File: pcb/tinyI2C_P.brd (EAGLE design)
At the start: 83.2 x 83.2 mm, 218 parts, among them IC1 IC_TTL_74_125, IC10 IC_TTL_74_125, IC11 TPS73618(0.4A), IC12 IC_TTL_74_125, IC13 TPS73618(0.4A), IC14 IC_TTL_74_125, IC15 TPS73618(0.4A), IC16 IC_TTL_74_125, IC2 TPS73618(0.4A), IC3 TPS73618(0.4A), IC4 IC_TTL_74_125, IC5 TPS73618(0.4A), IC6 IC_TTL_74_125, IC7 TPS73618(0.4A), IC8 IC_TTL_74_125, IC9 TPS73618(0.4A), U1 LPC824M201JHI33, U2 LPC824M201JHI33, U3 LPC824M201JHI33, U4 LPC824M201JHI33, U5 LPC824M201JHI33, U6 LPC824M201JHI33, U7 LPC824M201JHI33, U8 LPC824M201JHI33, X1 TSW-112-02-S-S, X10 TSW-102-02-S-S, X11 TSW-106-02-S-S-RA, X12 TSW-112-02-S-S, X13 TSW-112-02-S-S, X14 TSW-102-02-S-S, X15 TSW-102-02-S-S, X16 TSW-106-02-S-S-RA, X17 TSW-112-02-S-S, X18 TSW-112-02-S-S, X19 TSW-102-02-S-S, X2 TSW-106-02-S-S-RA, X20 TSW-102-02-S-S, X21 TSW-106-02-S-S-RA, X22 TSW-112-02-S-S, X23 TSW-112-02-S-S, X24 TSW-102-02-S-S, X25 TSW-102-02-S-S, X26 TSW-106-02-S-S-RA, X27 TSW-112-02-S-S, X28 TSW-112-02-S-S, X29 TSW-102-02-S-S, X3 TSW-112-02-S-S, X30 TSW-102-02-S-S, X31 TSW-106-02-S-S-RA, X32 TSW-112-02-S-S, X33 TSW-112-02-S-S, X34 TSW-102-02-S-S, X35 TSW-102-02-S-S, X36 TSW-106-02-S-S-RA, X37 TSW-112-02-S-S, X38 TSW-112-02-S-S, X39 TSW-102-02-S-S, X4 TSW-102-02-S-S, X40 TSW-102-02-S-S, X5 TSW-102-02-S-S, X6 TSW-106-02-S-S-RA, X7 TSW-112-02-S-S, X8 TSW-112-02-S-S, X9 TSW-102-02-S-S

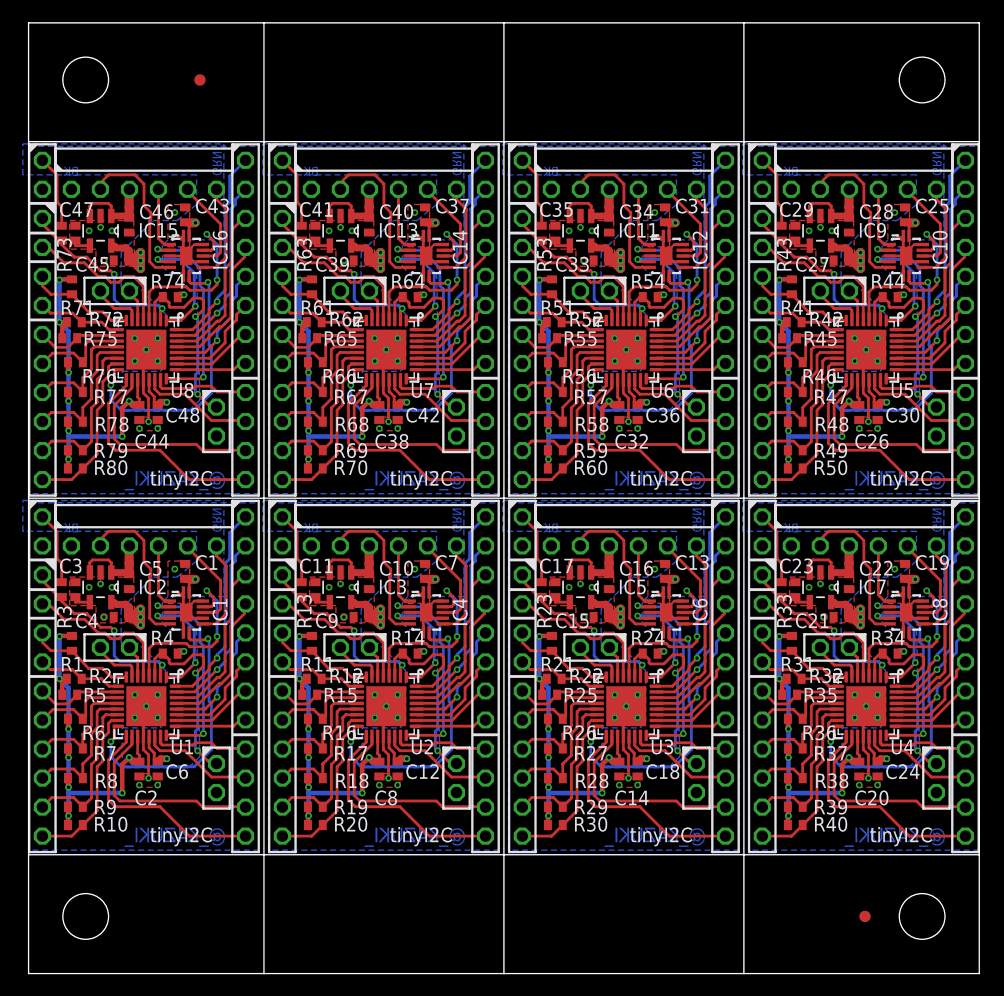
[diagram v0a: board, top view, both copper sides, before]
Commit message: [ PCB ] trace change and panelize
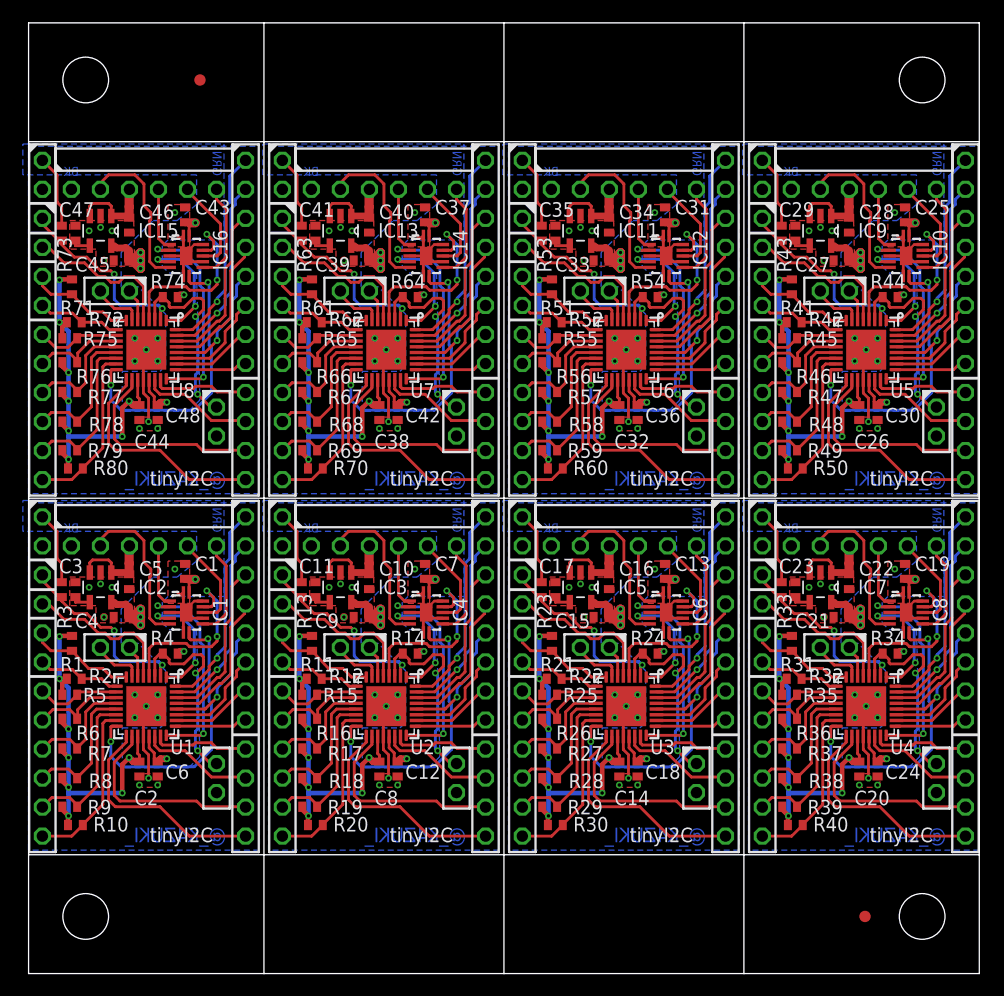
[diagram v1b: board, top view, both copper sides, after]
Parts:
- moved R16 0.50 mm to (24.6, 22.3)
- moved R17 0.50 mm to (24.6, 19.7)
- moved R18 0.50 mm to (24.6, 17.1)
- moved R19 0.50 mm to (24.6, 14.6)
- moved R26 0.50 mm to (45.6, 22.3)
- moved R27 0.50 mm to (45.6, 19.7)
- moved R28 0.50 mm to (45.6, 17.1)
- moved R29 0.50 mm to (45.6, 14.6)
- moved R36 0.50 mm to (66.6, 22.3)
- moved R37 0.50 mm to (66.6, 19.7)
- moved R38 0.50 mm to (66.6, 17.1)
- moved R39 0.50 mm to (66.6, 14.6)
- moved R46 0.50 mm to (66.6, 53.5)
- moved R47 0.50 mm to (66.6, 50.9)
- moved R48 0.50 mm to (66.6, 48.3)
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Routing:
- net 1.8V7: track 53.9 -> 54.7 mm
- net 1.8V6: track 53.9 -> 54.7 mm
- net 1.8V4: track 53.9 -> 54.7 mm
- net 1.8V5: track 53.9 -> 54.7 mm
- net 1.8V3: track 53.9 -> 54.7 mm
- net 1.8V2: track 53.9 -> 54.7 mm
- net 1.8V1: track 53.9 -> 54.7 mm
- net 1.8V: track 53.9 -> 54.7 mm

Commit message: [ PCB ] panelized based on sch/brd updates
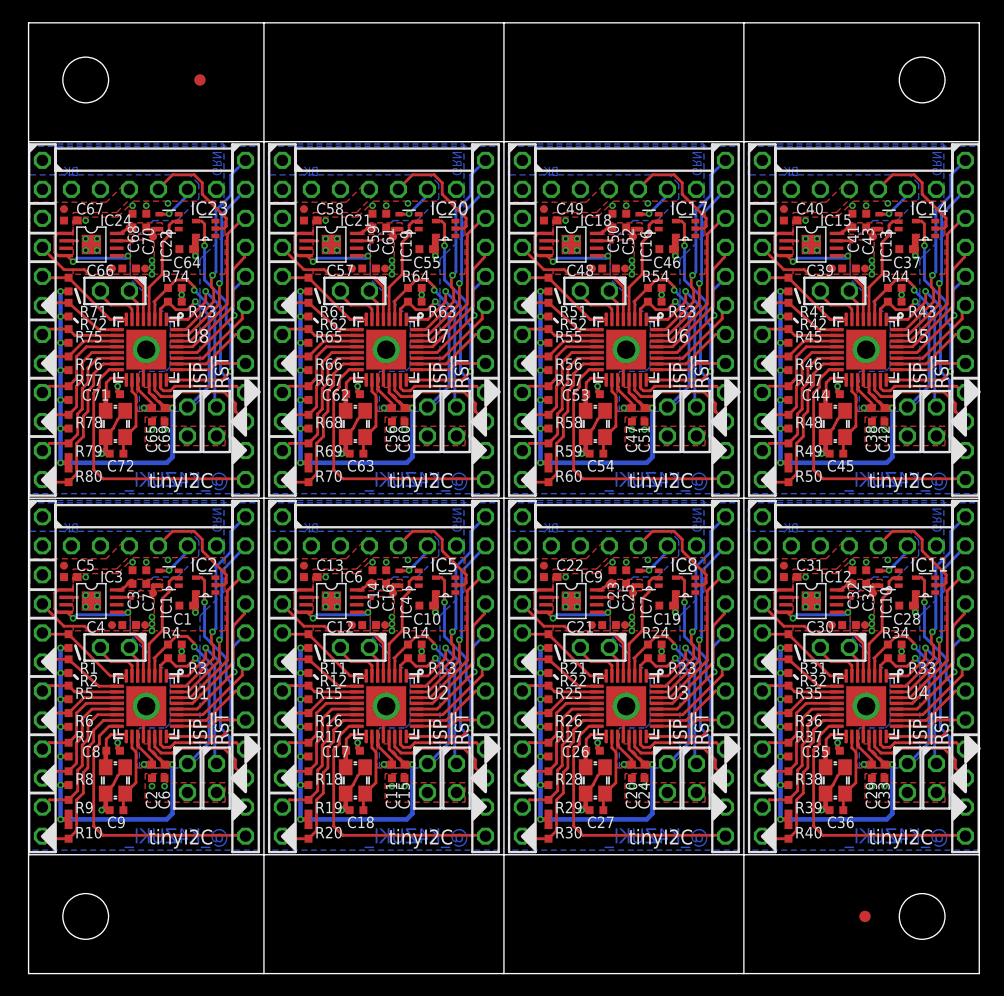
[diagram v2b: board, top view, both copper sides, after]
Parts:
- added C49, C50, C51, C52, C53, C54, C55, C56, C57, C58, C59, C60, C61, C62, C63, C64, C65, C66, C67, C68, C69, C70, C71, C72: 1005, mylib:C0402
- added IC17, IC19, IC20, IC22, IC23: 74LVC1G125DCK, 74xx-little-us_local:SC70-5
- added IC18, IC21, IC24: IC_LDO_MIC5355, mylib:IC_08_0.65_160MIL
- added Q1, Q2, Q3, Q4, Q5, Q6, Q7, Q8: (no value), adafruit (1):NX3225
- added TP27, TP28, TP29, TP30, TP31, TP32, TP33, TP34: TPTP07R, testpad_local:TP07R
- added X41, X42, X46, X47, X48: TSW-102-02-S-S, con-samtec.local:TSW-102-02-S-S
- added X43: TSW-106-02-S-S-RA, con-samtec.local:TSW-106-02-S-S-RA
- added X44, X45: TSW-112-02-S-S, con-samtec.local:TSW-112-02-S-S
- C1, C11, C12, C13, C14, C15, C17, C18, C19, C2, C20, C21, C23, C24, C25, C26, C27, C29, C3, C30, C31, C32, C33, C35, C36, C37, C38, C39, C4, C41, C42, C43, C44, C45, C47, C48, C6, C7, C8, C9: device rcl:C1005 -> mylib:C0402
- C10, C16, C22, C28, C34, C40, C46, C5: value 1608 -> 1005; device rcl:C0402 -> mylib:C0402
- IC1, IC10, IC14, IC16, IC4, IC8: value IC_TTL_74_125 -> 74LVC1G125DCK; device mylib:DHVQFN14 -> 74xx-little-us_local:SC70-5
- IC11, IC13, IC2, IC5, IC7: value TPS73618(0.4A) -> 74LVC1G125DCK; device mylib:SOT95P280X145-5N -> 74xx-little-us_local:SC70-5
- IC12, IC6: value IC_TTL_74_125 -> IC_LDO_MIC5355; device mylib:DHVQFN14 -> mylib:IC_08_0.65_160MIL
- IC15, IC3, IC9: value TPS73618(0.4A) -> IC_LDO_MIC5355; device mylib:SOT95P280X145-5N -> mylib:IC_08_0.65_160MIL
- R1, R10, R11, R12, R13, R14, R15, R16, R17, R18, R19, R2, R20, R21, R22, R23, R24, R25, R26, R27, R28, R29, R3, R30, R31, R32, R33, R34, R35, R36, R37, R38, R39, R4, R40, R41, R42, R43, R44, R45, R46, R47, R48, R49, R5, R50, R51, R52, R53, R54, R55, R56, R57, R58, R59, R6, R60, R61, R62, R63, R64, R65, R66, R67, R68, R69, R7, R70, R71, R72, R73, R74, R75, R76, R77, R78, R79, R8, R80, R9: device rcl:R1005 -> mylib:C0402
- TP1, TP10, TP11, TP12, TP13, TP14, TP15, TP16, TP17, TP18, TP19, TP2, TP20, TP21, TP22, TP23, TP24, TP25, TP26, TP3, TP6, TP7, TP8, TP9: device testpad:TP07R -> testpad_local:TP07R
- X11, X16, X36, X6: value TSW-106-02-S-S-RA -> TSW-102-02-S-S; device con-samtec.local:TSW-106-02-S-S-RA -> con-samtec.local:TSW-102-02-S-S
- X12, X17, X18, X22, X23, X28: value TSW-112-02-S-S -> TSW-102-02-S-S; device con-samtec.local:TSW-112-02-S-S -> con-samtec.local:TSW-102-02-S-S
- X13, X3, X37, X7: value TSW-112-02-S-S -> TSW-106-02-S-S-RA; device con-samtec.local:TSW-112-02-S-S -> con-samtec.local:TSW-106-02-S-S-RA
- X14, X15, X20, X39, X9: value TSW-102-02-S-S -> TSW-112-02-S-S; device con-samtec.local:TSW-102-02-S-S -> con-samtec.local:TSW-112-02-S-S
- X19, X25: value TSW-102-02-S-S -> TSW-106-02-S-S-RA; device con-samtec.local:TSW-102-02-S-S -> con-samtec.local:TSW-106-02-S-S-RA
- X2, X21, X26: value TSW-106-02-S-S-RA -> TSW-112-02-S-S; device con-samtec.local:TSW-106-02-S-S-RA -> con-samtec.local:TSW-112-02-S-S
- moved C45 64.8 mm to (70.7, 45.5)
- moved IC15 62.2 mm to (68.5, 63.8)
- moved C44 60.7 mm to (70.4, 50.7), turned to 0 degrees
- moved C43 59.6 mm to (73.3, 65.9)
- moved C27 52.6 mm to (49.7, 14.3)
- moved C35 51.4 mm to (70.4, 19.5), turned to 0 degrees
- moved C47 51.2 mm to (52.8, 48.9), turned to 270 degrees
- moved C33 51.1 mm to (74.9, 17.7), turned to 270 degrees
- moved X36 50.8 mm to (55.9, 48.3), turned to 90 degrees
- moved IC13 48.0 mm to (75.3, 65.8), turned to 90 degrees
- moved C29 47.6 mm to (73.8, 17.7), turned to 270 degrees
- moved C46 47.0 mm to (55.8, 63.4), turned to 180 degrees
- moved C41 47.0 mm to (72.1, 65.9)
- moved TP26 46.3 mm to (52.9, 64.5)
- moved X21 45.0 mm to (82.0, 26.0), turned to 90 degrees
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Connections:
- removed net CTS<-: IC1.6, X2.2
- removed net CTS<-1: IC4.6, X6.2
- removed net CTS<-2: IC6.6, X11.2
- removed net CTS<-3: IC8.6, X16.2
- removed net CTS<-4: IC10.6, X21.2
- removed net CTS<-5: IC12.6, X26.2
- removed net CTS<-6: IC14.6, X31.2
- removed net CTS<-7: IC16.6, X36.2
- removed net RTS->: IC1.9, X2.6
- removed net RTS->1: IC4.9, X6.6
- removed net RTS->2: IC6.9, X11.6
- removed net RTS->3: IC8.9, X16.6
- removed net RTS->4: IC10.9, X21.6
- removed net RTS->5: IC12.9, X26.6
- removed net RTS->6: IC14.9, X31.6
- removed net RTS->7: IC16.9, X36.6
- removed net TGT_CTS: IC1.8, U1.16
- removed net TGT_CTS1: IC4.8, U2.16
- removed net TGT_CTS2: IC6.8, U3.16
- removed net TGT_CTS3: IC8.8, U4.16
- removed net TGT_CTS4: IC10.8, U5.16
- removed net TGT_CTS5: IC12.8, U6.16
- removed net TGT_CTS6: IC14.8, U7.16
- removed net TGT_CTS7: IC16.8, U8.16
- removed net TGT_RTS: IC1.5, U1.1
- removed net TGT_RTS1: IC4.5, U2.1
- removed net TGT_RTS2: IC6.5, U3.1
- removed net TGT_RTS3: IC8.5, U4.1
- removed net TGT_RTS4: IC10.5, U5.1
- removed net TGT_RTS5: IC12.5, U6.1
- removed net TGT_RTS6: IC14.5, U7.1
- removed net TGT_RTS7: IC16.5, U8.1
- new net 3.3V: C3.1, C7.1, IC1.5, IC3.8, TP6.TP
- new net 3.3V1: C14.1, C16.1, IC4.5, IC6.8, TP10.TP
- new net 3.3V2: C23.1, C25.1, IC7.5, IC9.8, TP14.TP
- new net 3.3V3: C32.1, C34.1, IC10.5, IC12.8, TP18.TP
- new net 3.3V4: C41.1, C43.1, IC13.5, IC15.8, TP22.TP
- new net 3.3V5: C50.1, C52.1, IC16.5, IC18.8, TP26.TP
- new net 3.3V6: C59.1, C61.1, IC19.5, IC21.8, TP30.TP
- new net 3.3V7: C68.1, C70.1, IC22.5, IC24.8, TP34.TP
- new net N$10: C45.1, Q5.3, U5.18
- new net N$11: C53.1, Q6.1, U6.17
- new net N$12: C54.1, Q6.3, U6.18
- new net N$13: C62.1, Q7.1, U7.17
- new net N$14: C63.1, Q7.3, U7.18
- new net N$15: C71.1, Q8.1, U8.17
- new net N$16: C72.1, Q8.3, U8.18
- new net N$9: C44.1, Q5.1, U5.17
- net !ISP!: now also X6.1; no longer X1.3
- net !ISP!1: now also X12.1; no longer X7.3
- net !ISP!2: now also X18.1; no longer X12.3
- net !ISP!3: now also X24.1; no longer X17.3
- net !ISP!4: now also X30.1; no longer X22.3
- net !ISP!5: now also X36.1; no longer X27.3
- net !ISP!6: now also X42.1; no longer X32.3
- net !ISP!7: now also X48.1; no longer X37.3
- net !RESET!1: now also X10.1; no longer X9.1
- net !RESET!2: now also X16.1; no longer X14.1
- net !RESET!3: now also X22.1; no longer X19.1
- net !RESET!4: now also X28.1; no longer X24.1
- net !RESET!5: now also X34.1; no longer X29.1
- net !RESET!6: now also X40.1; no longer X34.1
- net !RESET!7: now also X46.1; no longer X39.1
- net 1.8V: now also IC3.7; no longer IC1.14
- net 1.8V1: now also C10.1, C11.1, C15.1, IC5.5, IC6.7, TP8.TP, X8.1; no longer C7.1, C8.1, C9.1, IC3.5, IC4.14, TP7.TP, X7.1
- net 1.8V2: now also C19.1, C20.1, C21.1, C24.1, IC8.5, IC9.7, TP12.TP, X14.1; no longer C13.1, C14.1, C15.1, C18.1, IC5.5, IC6.14, TP10.TP, X12.1
- net 1.8V3: now also C28.1, C29.1, C30.1, C33.1, IC11.5, IC12.7, TP16.TP, X20.1; no longer C19.1, C20.1, C21.1, C24.1, IC7.5, IC8.14, TP13.TP, X17.1
- net 1.8V4: now also C37.1, C38.1, C39.1, C42.1, IC14.5, IC15.7, TP20.TP, X26.1; no longer C25.1, C26.1, C27.1, C30.1, IC10.14, IC9.5, TP16.TP, X22.1
- net 1.8V5: now also C46.1, C47.1, C48.1, C51.1, IC17.5, IC18.7, TP24.TP, X32.1; no longer C31.1, C32.1, C33.1, C36.1, IC11.5, IC12.14, TP19.TP, X27.1
- net 1.8V6: now also C55.1, C56.1, C57.1, C60.1, IC20.5, IC21.7, TP28.TP, X38.1; no longer C37.1, C38.1, C39.1, C42.1, IC13.5, IC14.14, TP22.TP, X32.1
- net 1.8V7: now also C64.1, C65.1, C66.1, C69.1, IC23.5, IC24.7, TP32.TP, X44.1; no longer C43.1, C44.1, C45.1, C48.1, IC15.5, IC16.14, TP25.TP, X37.1
- net 5V: now also IC3.1, IC3.4, IC3.5, X1.3, X3.3; no longer IC2.1, IC2.3, X2.3
- net 5V1: now also C13.1, IC6.1, IC6.4, IC6.5, TP7.TP, X7.3, X8.3; no longer C10.1, IC3.1, IC3.3, TP6.TP, X6.3
- net 5V2: now also C22.1, IC9.1, IC9.4, IC9.5, TP11.TP, X13.3, X14.3; no longer C16.1, IC5.1, IC5.3, TP9.TP, X11.3
- net 5V3: now also C31.1, IC12.1, IC12.4, IC12.5, TP15.TP, X19.3, X20.3; no longer C22.1, IC7.1, IC7.3, TP12.TP, X16.3
- net 5V4: now also C40.1, IC15.1, IC15.4, IC15.5, TP19.TP, X25.3, X26.3; no longer C28.1, IC9.1, IC9.3, TP15.TP, X21.3
- net 5V5: now also C49.1, IC18.1, IC18.4, IC18.5, TP23.TP, X31.3, X32.3; no longer C34.1, IC11.1, IC11.3, TP18.TP, X26.3
- net 5V6: now also C58.1, IC21.1, IC21.4, IC21.5, TP27.TP, X37.3, X38.3; no longer C40.1, IC13.1, IC13.3, TP21.TP, X31.3
- net 5V7: now also C67.1, IC24.1, IC24.4, IC24.5, TP31.TP, X43.3, X44.3; no longer C46.1, IC15.1, IC15.3, TP24.TP, X36.3
- net GND: now also C7.2, C8.2, C9.2, IC1.3, IC2.1, IC2.3, IC3.2, IC3.EXP, Q1.2, Q1.4, X3.1, X6.2; no longer IC1.10, IC1.13, IC1.4, IC1.7, IC1.EXP, IC2.2, X2.1
- net GND1: now also C13.2, C14.2, C15.2, C16.2, C17.2, C18.2, IC4.3, IC5.1, IC5.3, IC6.2, IC6.EXP, Q2.2, Q2.4, TP9.TP, X10.2, X12.2, X7.1, X8.2; no longer C7.2, C8.2, C9.2, IC3.2, IC4.10, IC4.13, IC4.4, IC4.7, IC4.EXP, TP8.TP, X6.1, X7.2, X9.2
- net GND2: now also C19.2, C20.2, C21.2, C22.2, C23.2, C24.2, C25.2, C26.2, C27.2, IC7.1, IC7.3, IC8.1, IC8.3, IC9.2, IC9.EXP, Q3.2, Q3.4, TP13.TP, X13.1, X16.2, X18.2; no longer C13.2, C14.2, C15.2, C16.2, C17.2, C18.2, IC5.2, IC6.1, IC6.10, IC6.13, IC6.4, IC6.7, IC6.EXP, TP11.TP, X11.1, X12.2
- net GND3: now also C28.2, C29.2, C30.2, C31.2, C32.2, C33.2, C34.2, C35.2, C36.2, IC10.1, IC10.3, IC11.1, IC11.3, IC12.2, IC12.EXP, Q4.2, Q4.4, TP17.TP, X19.1, X20.2, X22.2, X24.2; no longer C19.2, C20.2, C21.2, C22.2, C23.2, C24.2, IC7.2, IC8.1, IC8.10, IC8.13, IC8.4, IC8.7, IC8.EXP, TP14.TP, X16.1, X17.2, X19.2
- net GND4: now also C37.2, C38.2, C39.2, C40.2, C41.2, C42.2, C43.2, C44.2, C45.2, IC13.1, IC13.3, IC14.1, IC14.3, IC15.2, IC15.EXP, Q5.2, Q5.4, TP21.TP, X25.1, X26.2, X28.2, X30.2; no longer C25.2, C26.2, C27.2, C28.2, C29.2, C30.2, IC10.1, IC10.10, IC10.13, IC10.4, IC10.7, IC10.EXP, IC9.2, TP17.TP, X21.1, X22.2, X24.2
- net GND5: now also C46.2, C47.2, C48.2, C49.2, C50.2, C51.2, C52.2, C53.2, C54.2, IC16.1, IC16.3, IC17.1, IC17.3, IC18.2, IC18.EXP, Q6.2, Q6.4, TP25.TP, X31.1, X32.2, X34.2, X36.2; no longer C31.2, C32.2, C33.2, C34.2, C35.2, C36.2, IC11.2, IC12.1, IC12.10, IC12.13, IC12.4, IC12.7, IC12.EXP, TP20.TP, X26.1, X27.2, X29.2
- net GND6: now also C55.2, C56.2, C57.2, C58.2, C59.2, C60.2, C61.2, C62.2, C63.2, IC19.1, IC19.3, IC20.1, IC20.3, IC21.2, IC21.EXP, Q7.2, Q7.4, TP29.TP, X37.1, X38.2, X40.2, X42.2; no longer C37.2, C38.2, C39.2, C40.2, C41.2, C42.2, IC13.2, IC14.1, IC14.10, IC14.13, IC14.4, IC14.7, IC14.EXP, TP23.TP, X31.1, X32.2, X34.2
- net GND7: now also C64.2, C65.2, C66.2, C67.2, C68.2, C69.2, C70.2, C71.2, C72.2, IC22.1, IC22.3, IC23.1, IC23.3, IC24.2, IC24.EXP, Q8.2, Q8.4, TP33.TP, X43.1, X44.2, X46.2, X48.2; no longer C43.2, C44.2, C45.2, C46.2, C47.2, C48.2, IC15.2, IC16.1, IC16.10, IC16.13, IC16.4, IC16.7, IC16.EXP, TP26.TP, X36.1, X37.2, X39.2
- net GPIO00: now also X2.1; no longer X3.1
- net GPIO01: now also X2.2; no longer X3.2
- net GPIO02: now also X2.3; no longer X3.3
- net GPIO03: now also X2.4; no longer X3.4
- net GPIO04: now also X2.5; no longer X3.5
- net GPIO05: now also X2.6; no longer X3.6
- net GPIO06: now also X2.7; no longer X3.7
- net GPIO07: now also X2.8; no longer X3.8
- net GPIO08: now also X8.4; no longer X7.4
- net GPIO09: now also X8.7; no longer X7.7
- net GPIO100: now also X39.5; no longer X33.5
- net GPIO101: now also X39.4; no longer X33.4
- net GPIO102: now also X39.3; no longer X33.3
- net GPIO103: now also X39.2; no longer X33.2
- net GPIO104: now also X39.1; no longer X33.1
- net GPIO105: now also X44.4; no longer X37.4
- net GPIO106: now also X44.7; no longer X37.7
- net GPIO107: now also X44.8; no longer X37.8
- net GPIO108: now also X44.9; no longer X37.9
- net GPIO109: now also X44.10; no longer X37.10
- net GPIO110: now also X44.11; no longer X37.11
- net GPIO111: now also X44.12; no longer X37.12
- net GPIO112: now also X45.8; no longer X38.8
- net GPIO113: now also X45.7; no longer X38.7
- net GPIO114: now also X45.6; no longer X38.6
- net GPIO115: now also X45.5; no longer X38.5
- net GPIO116: now also X45.4; no longer X38.4
- net GPIO117: now also X45.3; no longer X38.3
- net GPIO118: now also X45.2; no longer X38.2
- net GPIO119: now also X45.1; no longer X38.1
- net GPIO17: now also X8.8; no longer X7.8
- net GPIO18: now also X8.9; no longer X7.9
- net GPIO19: now also X8.10; no longer X7.10
- net GPIO20: now also X8.11; no longer X7.11
- net GPIO21: now also X8.12; no longer X7.12
- net GPIO22: now also X9.8; no longer X8.8
- net GPIO23: now also X9.7; no longer X8.7
- net GPIO24: now also X9.6; no longer X8.6
- net GPIO25: now also X9.5; no longer X8.5
- net GPIO26: now also X9.4; no longer X8.4
- net GPIO27: now also X9.3; no longer X8.3
- net GPIO28: now also X9.2; no longer X8.2
- net GPIO29: now also X9.1; no longer X8.1
- net GPIO30: now also X14.4; no longer X12.4
- net GPIO31: now also X14.7; no longer X12.7
- net GPIO32: now also X14.8; no longer X12.8
- net GPIO33: now also X14.9; no longer X12.9
- net GPIO34: now also X14.10; no longer X12.10
- net GPIO35: now also X14.11; no longer X12.11
- net GPIO36: now also X14.12; no longer X12.12
- net GPIO37: now also X15.8; no longer X13.8
- net GPIO38: now also X15.7; no longer X13.7
- net GPIO39: now also X15.6; no longer X13.6
- net GPIO40: now also X15.5; no longer X13.5
- net GPIO41: now also X15.4; no longer X13.4
- net GPIO42: now also X15.3; no longer X13.3
- net GPIO43: now also X15.2; no longer X13.2
- net GPIO44: now also X15.1; no longer X13.1
- net GPIO45: now also X20.4; no longer X17.4
- net GPIO46: now also X20.7; no longer X17.7
- net GPIO47: now also X20.8; no longer X17.8
- net GPIO48: now also X20.9; no longer X17.9
- net GPIO49: now also X20.10; no longer X17.10
- net GPIO50: now also X20.11; no longer X17.11
- net GPIO51: now also X20.12; no longer X17.12
- net GPIO52: now also X21.8; no longer X18.8
- net GPIO53: now also X21.7; no longer X18.7
- net GPIO54: now also X21.6; no longer X18.6
- net GPIO55: now also X21.5; no longer X18.5
- net GPIO56: now also X21.4; no longer X18.4
- net GPIO57: now also X21.3; no longer X18.3
- net GPIO58: now also X21.2; no longer X18.2
- net GPIO59: now also X21.1; no longer X18.1
- net GPIO60: now also X26.4; no longer X22.4
- net GPIO61: now also X26.7; no longer X22.7
- net GPIO62: now also X26.8; no longer X22.8
- net GPIO63: now also X26.9; no longer X22.9
- net GPIO64: now also X26.10; no longer X22.10
- net GPIO65: now also X26.11; no longer X22.11
- net GPIO66: now also X26.12; no longer X22.12
- net GPIO67: now also X27.8; no longer X23.8
- net GPIO68: now also X27.7; no longer X23.7
- net GPIO69: now also X27.6; no longer X23.6
- net GPIO70: now also X27.5; no longer X23.5
- net GPIO71: now also X27.4; no longer X23.4
- net GPIO72: now also X27.3; no longer X23.3
- net GPIO73: now also X27.2; no longer X23.2
- net GPIO74: now also X27.1; no longer X23.1
- net GPIO75: now also X32.4; no longer X27.4
- net GPIO76: now also X32.7; no longer X27.7
- net GPIO77: now also X32.8; no longer X27.8
- net GPIO78: now also X32.9; no longer X27.9
- net GPIO79: now also X32.10; no longer X27.10
- net GPIO80: now also X32.11; no longer X27.11
- net GPIO81: now also X32.12; no longer X27.12
- net GPIO82: now also X33.8; no longer X28.8
- net GPIO83: now also X33.7; no longer X28.7
- net GPIO84: now also X33.6; no longer X28.6
- net GPIO85: now also X33.5; no longer X28.5
- net GPIO86: now also X33.4; no longer X28.4
- net GPIO87: now also X33.3; no longer X28.3
- net GPIO88: now also X33.2; no longer X28.2
- net GPIO89: now also X33.1; no longer X28.1
- net GPIO90: now also X38.4; no longer X32.4
- net GPIO91: now also X38.7; no longer X32.7
- net GPIO92: now also X38.8; no longer X32.8
- net GPIO93: now also X38.9; no longer X32.9
- net GPIO94: now also X38.10; no longer X32.10
- net GPIO95: now also X38.11; no longer X32.11
- net GPIO96: now also X38.12; no longer X32.12
- net GPIO97: now also X39.8; no longer X33.8
- net GPIO98: now also X39.7; no longer X33.7
- net GPIO99: now also X39.6; no longer X33.6
- net I2C_SCL1: now also X8.6; no longer X7.6
- net I2C_SCL2: now also X14.6; no longer X12.6
- net I2C_SCL3: now also X20.6; no longer X17.6
- net I2C_SCL4: now also X26.6; no longer X22.6
- net I2C_SCL5: now also X32.6; no longer X27.6
- net I2C_SCL6: now also X38.6; no longer X32.6
- net I2C_SCL7: now also X44.6; no longer X37.6
- net I2C_SDA1: now also X8.5; no longer X7.5
- net I2C_SDA2: now also X14.5; no longer X12.5
- net I2C_SDA3: now also X20.5; no longer X17.5
- net I2C_SDA4: now also X26.5; no longer X22.5
- net I2C_SDA5: now also X32.5; no longer X27.5
- net I2C_SDA6: now also X38.5; no longer X32.5
- net I2C_SDA7: now also X44.5; no longer X37.5
- net N$1: now also C8.1, Q1.1, U1.17; no longer C3.1, IC2.4
- net N$2: now also C17.1, Q2.1, U2.17; no longer C11.1, IC3.4
- net N$3: now also C9.1, Q1.3, U1.18; no longer C17.1, IC5.4
- net N$4: now also C18.1, Q2.3, U2.18; no longer C23.1, IC7.4
- net N$5: now also C26.1, Q3.1, U3.17; no longer C29.1, IC9.4
- net N$6: now also C27.1, Q3.3, U3.18; no longer C35.1, IC11.4
- net N$7: now also C35.1, Q4.1, U4.17; no longer C41.1, IC13.4
- net N$8: now also C36.1, Q4.3, U4.18; no longer C47.1, IC15.4
- net RX<-: now also IC1.4, X3.5; no longer IC1.11, X2.5
- net RX<-1: now also IC4.4, X7.5; no longer IC4.11, X6.5
- net RX<-2: now also IC7.4, X13.5; no longer IC6.11, X11.5
- net RX<-3: now also IC10.4, X19.5; no longer IC8.11, X16.5
- net RX<-4: now also IC13.4, X25.5; no longer IC10.11, X21.5
- net RX<-5: now also IC16.4, X31.5; no longer IC12.11, X26.5
- net RX<-6: now also IC19.4, X37.5; no longer IC14.11, X31.5
- net RX<-7: now also IC22.4, X43.5; no longer IC16.11, X36.5
- net SPI_CS: now also U1.16, X2.12; no longer U1.17, X3.12
- net SPI_CS1: now also U2.16, X9.12; no longer U2.17, X8.12
- net SPI_CS2: now also U3.16, X15.12; no longer U3.17, X13.12
- net SPI_CS3: now also U4.16, X21.12; no longer U4.17, X18.12
- net SPI_CS4: now also U5.16, X27.12; no longer U5.17, X23.12
- net SPI_CS5: now also U6.16, X33.12; no longer U6.17, X28.12
- net SPI_CS6: now also U7.16, X39.12; no longer U7.17, X33.12
- net SPI_CS7: now also U8.16, X45.12; no longer U8.17, X38.12
- net SPI_MISO: now also X2.10; no longer X3.10
- net SPI_MISO1: now also X9.10; no longer X8.10
- net SPI_MISO2: now also X15.10; no longer X13.10
- net SPI_MISO3: now also X21.10; no longer X18.10
- net SPI_MISO4: now also X27.10; no longer X23.10
- net SPI_MISO5: now also X33.10; no longer X28.10
- net SPI_MISO6: now also X39.10; no longer X33.10
- net SPI_MISO7: now also X45.10; no longer X38.10
- net SPI_MOSI: now also X2.9; no longer X3.9
- net SPI_MOSI1: now also X9.9; no longer X8.9
- net SPI_MOSI2: now also X15.9; no longer X13.9
- net SPI_MOSI3: now also X21.9; no longer X18.9
- net SPI_MOSI4: now also X27.9; no longer X23.9
- net SPI_MOSI5: now also X33.9; no longer X28.9
- net SPI_MOSI6: now also X39.9; no longer X33.9
- net SPI_MOSI7: now also X45.9; no longer X38.9
- net SPI_SCK: now also U1.1, X2.11; no longer U1.18, X3.11
- net SPI_SCK1: now also U2.1, X9.11; no longer U2.18, X8.11
- net SPI_SCK2: now also U3.1, X15.11; no longer U3.18, X13.11
- net SPI_SCK3: now also U4.1, X21.11; no longer U4.18, X18.11
- net SPI_SCK4: now also U5.1, X27.11; no longer U5.18, X23.11
- net SPI_SCK5: now also U6.1, X33.11; no longer U6.18, X28.11
- net SPI_SCK6: now also U7.1, X39.11; no longer U7.18, X33.11
- net SPI_SCK7: now also U8.1, X45.11; no longer U8.18, X38.11
- net SWCLK1: now also X11.1; no longer X10.1
- net SWCLK2: now also X17.1; no longer X15.1
- net SWCLK3: now also X23.1; no longer X20.1
- net SWCLK4: now also X29.1; no longer X25.1
- net SWCLK5: now also X35.1; no longer X30.1
- net SWCLK6: now also X41.1; no longer X35.1
- net SWCLK7: now also X47.1; no longer X40.1
- net SWDIO1: now also X11.2; no longer X10.2
- net SWDIO2: now also X17.2; no longer X15.2
- net SWDIO3: now also X23.2; no longer X20.2
- net SWDIO4: now also X29.2; no longer X25.2
- net SWDIO5: now also X35.2; no longer X30.2
- net SWDIO6: now also X41.2; no longer X35.2
- net SWDIO7: now also X47.2; no longer X40.2
- net TGT_RX: now also IC2.4; no longer IC1.3
- net TGT_RX1: now also IC5.4; no longer IC4.3
- net TGT_RX2: now also IC8.4; no longer IC6.3
- net TGT_RX3: now also IC11.4; no longer IC8.3
- net TGT_RX4: now also IC14.4; no longer IC10.3
- net TGT_RX5: now also IC17.4; no longer IC12.3
- net TGT_RX6: now also IC20.4; no longer IC14.3
- net TGT_RX7: now also IC23.4; no longer IC16.3
- net TGT_TX: now also IC1.2; no longer IC1.12
- net TGT_TX1: now also IC4.2; no longer IC4.12
- net TGT_TX2: now also IC7.2; no longer IC6.12
- net TGT_TX3: now also IC10.2; no longer IC8.12
- net TGT_TX4: now also IC13.2; no longer IC10.12
- net TGT_TX5: now also IC16.2; no longer IC12.12
- net TGT_TX6: now also IC19.2; no longer IC14.12
- net TGT_TX7: now also IC22.2; no longer IC16.12
- net TX->: now also IC2.2, X3.4; no longer IC1.2, X2.4
- net TX->1: now also IC5.2, X7.4; no longer IC4.2, X6.4
- net TX->2: now also IC8.2, X13.4; no longer IC6.2, X11.4
- net TX->3: now also IC11.2, X19.4; no longer IC8.2, X16.4
- net TX->4: now also IC14.2, X25.4; no longer IC10.2, X21.4
- net TX->5: now also IC17.2, X31.4; no longer IC12.2, X26.4
- net TX->6: now also IC20.2, X37.4; no longer IC14.2, X31.4
- net TX->7: now also IC23.2, X43.4; no longer IC16.2, X36.4
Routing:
- net TGT_CTS1: track 25.0 -> 0.00 mm, vias 2 -> 0
- net TGT_CTS7: track 25.0 -> 0.00 mm, vias 2 -> 0
- net TGT_CTS6: track 25.0 -> 0.00 mm, vias 2 -> 0
- net TGT_CTS5: track 25.0 -> 0.00 mm, vias 2 -> 0
- net TGT_CTS3: track 25.0 -> 0.00 mm, vias 2 -> 0
- net TGT_CTS2: track 25.0 -> 0.00 mm, vias 2 -> 0
- net TGT_CTS4: track 25.0 -> 0.00 mm, vias 2 -> 0
- net TGT_CTS: track 25.0 -> 0.00 mm, vias 2 -> 0
- net CTS<-4: track 14.0 -> 0.00 mm
- net CTS<-5: track 14.0 -> 0.00 mm
- net CTS<-7: track 14.0 -> 0.00 mm
- net CTS<-6: track 14.0 -> 0.00 mm
- net CTS<-2: track 14.0 -> 0.00 mm
- net CTS<-3: track 14.0 -> 0.00 mm
- net CTS<-1: track 14.0 -> 0.00 mm
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- added copper zone on layer 1, net 1.8V
- added copper zone on layer 1, net 1.8V1
- added copper zone on layer 1, net 1.8V2
- added copper zone on layer 1, net 1.8V3
- added copper zone on layer 1, net 1.8V4
- added copper zone on layer 1, net 1.8V5
- added copper zone on layer 1, net 1.8V6
- added copper zone on layer 1, net 1.8V7
- added copper zone on layer 1, net 3.3V
- added copper zone on layer 1, net 3.3V1
- added copper zone on layer 1, net 3.3V2
- added copper zone on layer 1, net 3.3V3
- added copper zone on layer 1, net 3.3V4
- added copper zone on layer 1, net 3.3V5
- added copper zone on layer 1, net 3.3V6
- added copper zone on layer 1, net 3.3V7
- added copper zone on layer 1, net 5V
- added copper zone on layer 1, net 5V1
- added copper zone on layer 1, net 5V2
- added copper zone on layer 1, net 5V3
- added copper zone on layer 1, net 5V4
- added copper zone on layer 1, net 5V5
- added copper zone on layer 1, net 5V6
- added copper zone on layer 1, net 5V7
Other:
- board text added: "!ISP"
- board text added: "!RST"
- board text added: "C7"
- board text added: "C8"
- board text added: "C9"
- board text added: "IC3"
